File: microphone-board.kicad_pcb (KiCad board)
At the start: 4 copper layers, 10.7 x 11 mm, 13 parts, among them J1 Conn_FFC_Molex_5019510550

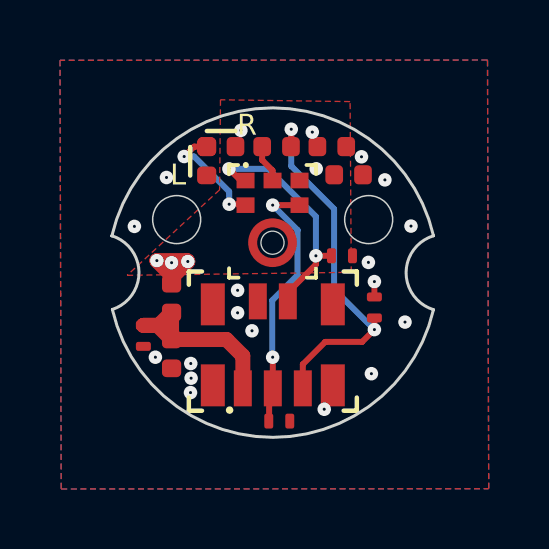
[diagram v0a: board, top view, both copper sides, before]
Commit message: [#72278] Route connections
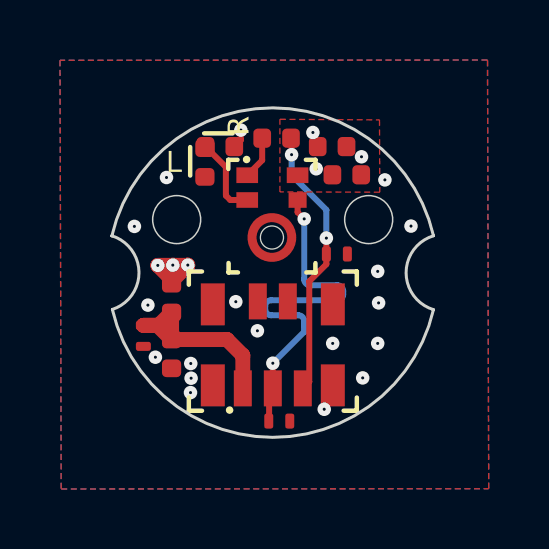
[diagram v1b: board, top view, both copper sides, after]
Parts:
- removed D3: TPD1E0B04_XDFN-2, antmicro-footprints:XDFN-2_1x0.60mm
- MK1: value MK_SPH0645LM4H-B -> MK_SPH0644LM4H-1; footprint antmicro-footprints:MK_SPH0645LM4H-B -> antmicro-footprints:MK_SPH0644LM4H-1
- moved D4 2.18 mm to (242.1, 146.3), turned to 0 degrees
- moved MK1 0.88 mm to (240.0, 145.0)
- moved R1 0.28 mm to (240.1, 142.4)
- moved R3 0.08 mm to (237.7, 143.2)
- moved C1 0.06 mm to (242.4, 143.7)
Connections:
- net /BCLK renamed /CLK
- J1 pad 4: /WS -> GND
- MK1 pad 1: /WS -> Net-(MK1-DATA)
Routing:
- net /WS: track 8.01 -> 0.00 mm, vias 2 -> 0
- net /CLK: track 8.91 -> 12.6 mm
- net /DATA: track 12.5 -> 9.08 mm
- net /SELECT: track 3.85 -> 2.69 mm, vias 2 -> 0
- net GND: track 0.62 -> 0.10 mm, vias 17 -> 18
